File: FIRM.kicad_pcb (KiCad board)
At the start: 4 copper layers, 21.1 x 26.9 mm, 99 parts, among them J1 DM3CS-SF, J2 Conn_01x02_Pin, Q1 IRLML6402, U1 W25Q128JVS, U2 STM32F405RGTx, U3 ADXL371, U5 INA219AxDCN, U6 MIC5219-3.3YM5, U9 A-USBC-20F0-EA-GSR05, X1 32.768khz, Y1 12 MHz

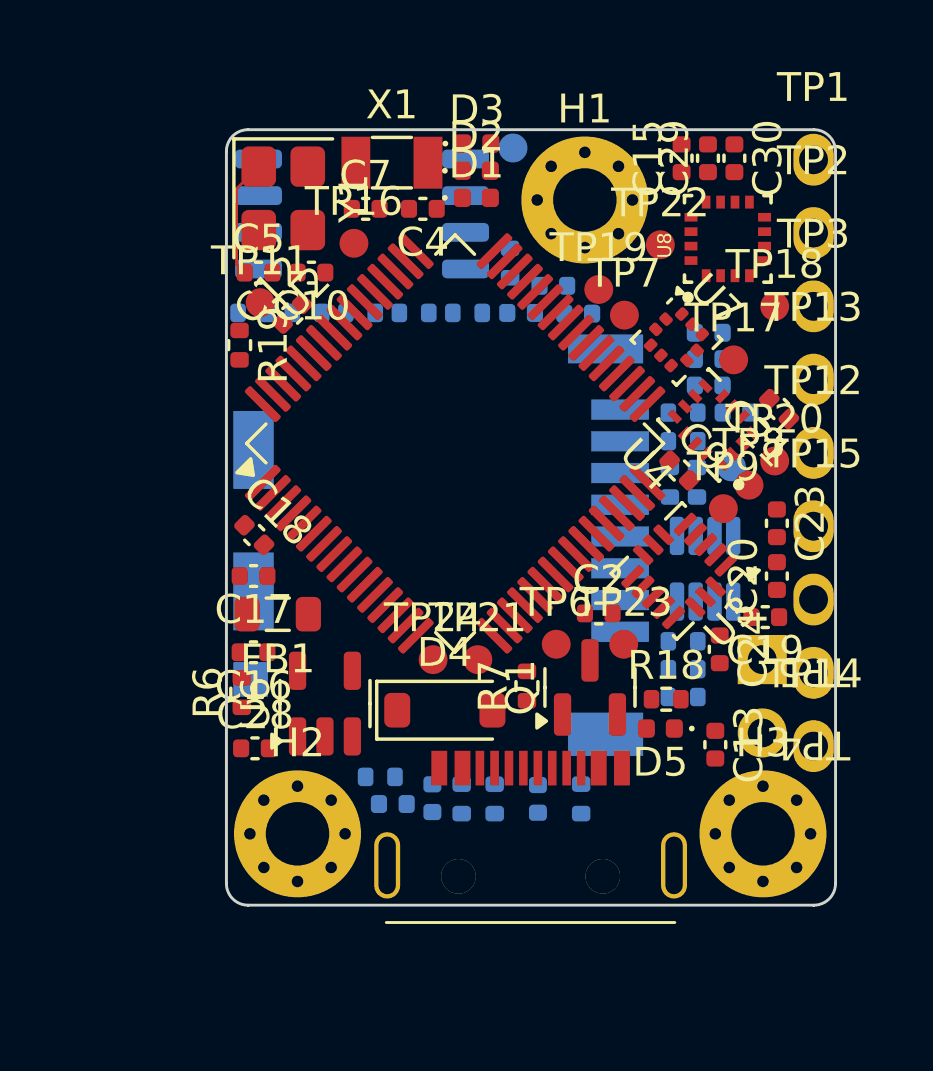
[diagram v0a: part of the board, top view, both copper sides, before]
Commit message: finished routing
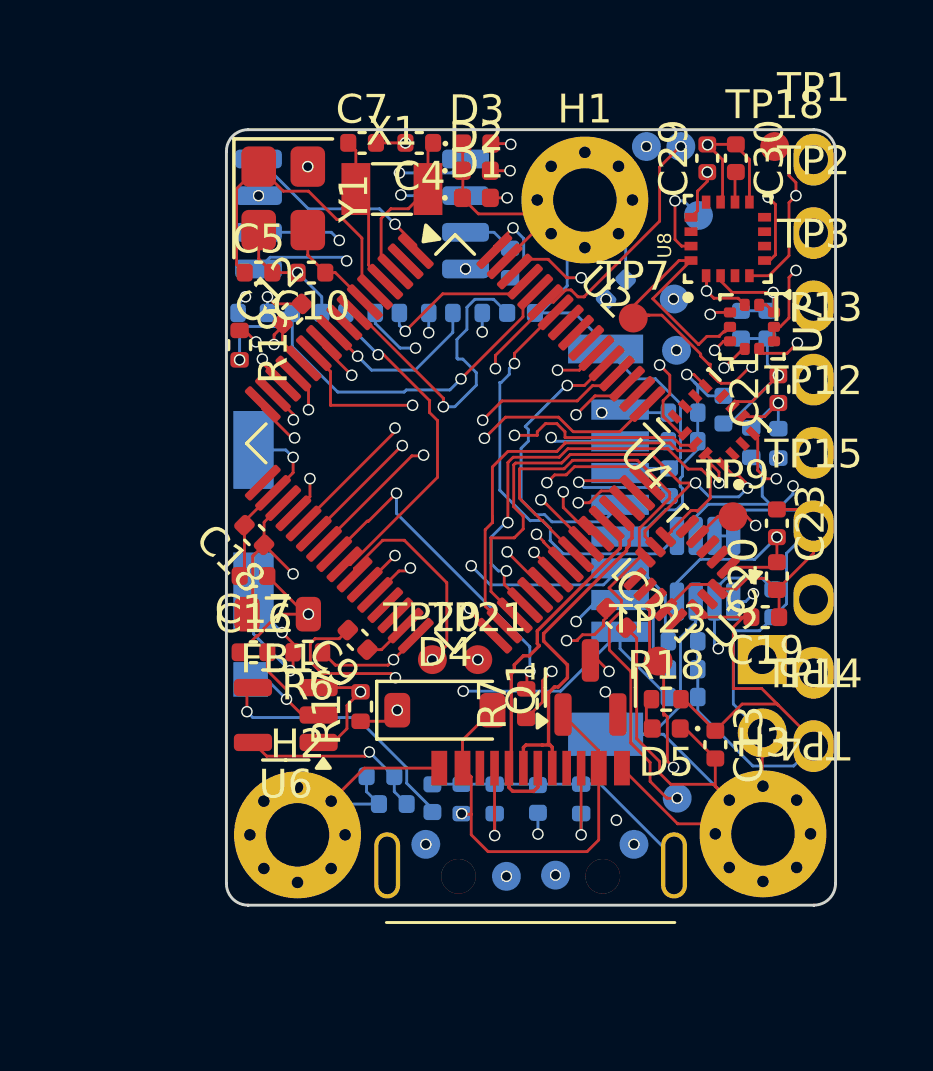
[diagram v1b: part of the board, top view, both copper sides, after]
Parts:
- removed C3, C6: 100n, Capacitor_SMD:C_0402_1005Metric
- C15, C24, C28, TP11, TP16, TP17, TP19, TP22, TP24, TP6, TP8: moved to B.Cu
- R17: moved to F.Cu
- moved TP25 25.2 mm to (163.1, 100.5)
- moved TP16 23.0 mm to (167.5, 99.4), turned to 180 degrees
- moved TP19 17.8 mm to (169.0, 97.8), turned to 180 degrees
- moved TP11 15.6 mm to (169.1, 75.3), turned to 180 degrees
- moved TP20 13.7 mm to (160.5, 93.0)
- moved C9 12.6 mm to (157.9, 92.4), turned to 135 degrees
- moved TP10 11.5 mm to (167.9, 75.3)
- moved TP24 8.59 mm to (164.8, 100.5), turned to 180 degrees
- moved TP6 8.28 mm to (160.3, 99.4), turned to 180 degrees
- moved TP8 6.95 mm to (168.9, 80.5), turned to 180 degrees
- moved C14 6.64 mm to (168.7, 86.9), turned to 90 degrees
- moved TP18 5.54 mm to (172.4, 75.3)
- moved C15 5.09 mm to (166.9, 80.2), turned to 45 degrees
- moved C28 4.45 mm to (158.7, 97.1), turned to 180 degrees
- moved R11 3.99 mm to (172.5, 85.5)
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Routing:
- net GND: track 0.00 -> 151.0 mm, vias 0 -> 12
- net +3.3V: track 0.00 -> 92.8 mm, vias 0 -> 17
- net /SCK2: track 0.00 -> 49.8 mm, vias 0 -> 3
- net /MISO2: track 0.00 -> 40.4 mm, vias 0 -> 5
- net /IMU_CS: track 0.00 -> 39.1 mm, vias 0 -> 3
- net /MOSI2: track 0.00 -> 37.8 mm, vias 0 -> 4
- net /I2C1_SCL: track 0.00 -> 35.1 mm, vias 0 -> 3
- net /BMP_INT: track 0.00 -> 31.5 mm, vias 0 -> 3
- net /I2C1_SDA: track 0.00 -> 31.0 mm, vias 0 -> 3
- net /NRST: track 0.00 -> 29.5 mm, vias 0 -> 2
- net /FLASH_CS: track 0.00 -> 27.1 mm, vias 0 -> 3
- net /MAG_CS: track 0.00 -> 25.8 mm, vias 0 -> 2
- net /IMU_INT: track 0.00 -> 25.7 mm, vias 0 -> 2
- net Net-(R19-Pad1): track 0.00 -> 24.2 mm, vias 0 -> 2
- net /SDIO_D2: track 0.00 -> 23.5 mm, vias 0 -> 2
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- added copper zone on In2.Cu, net +3.3V
- added copper zone on In1.Cu, net GND
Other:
- copper layers 4 -> 8

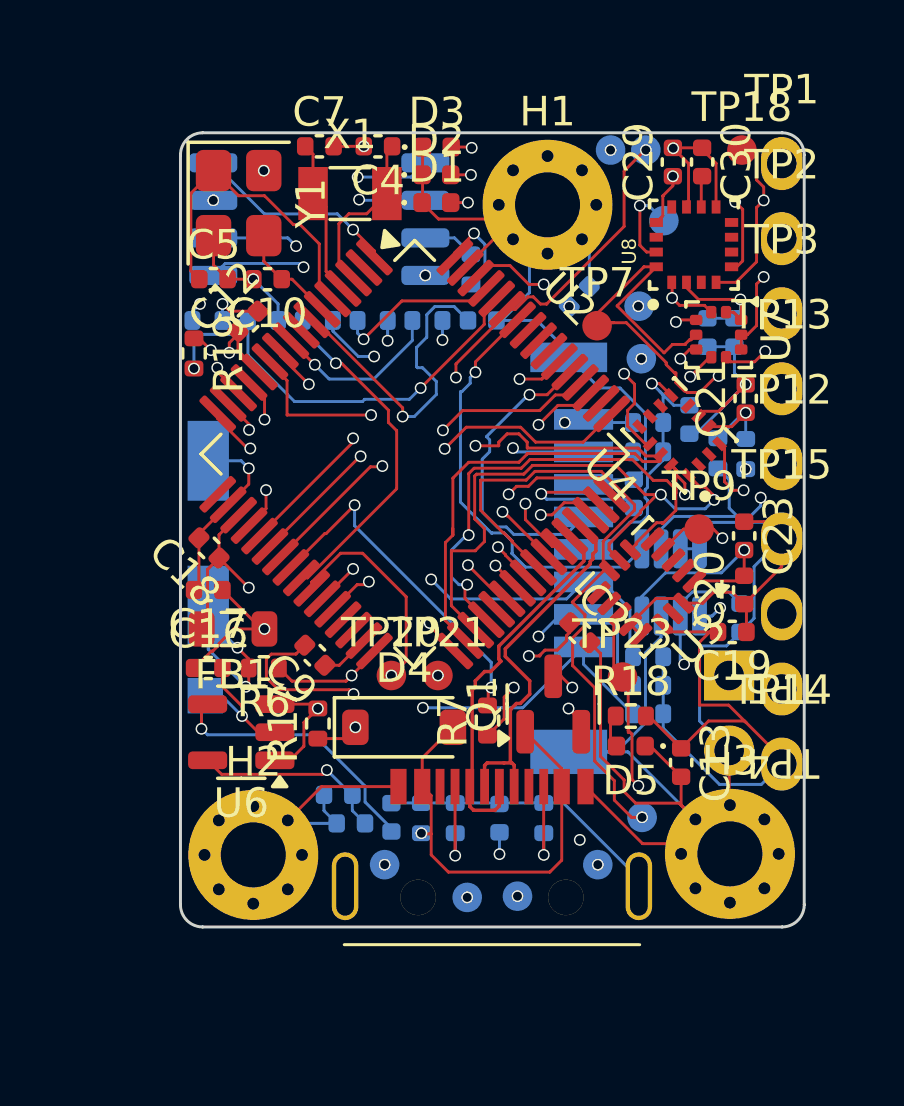
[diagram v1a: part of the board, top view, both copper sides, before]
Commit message: byebye drc errors
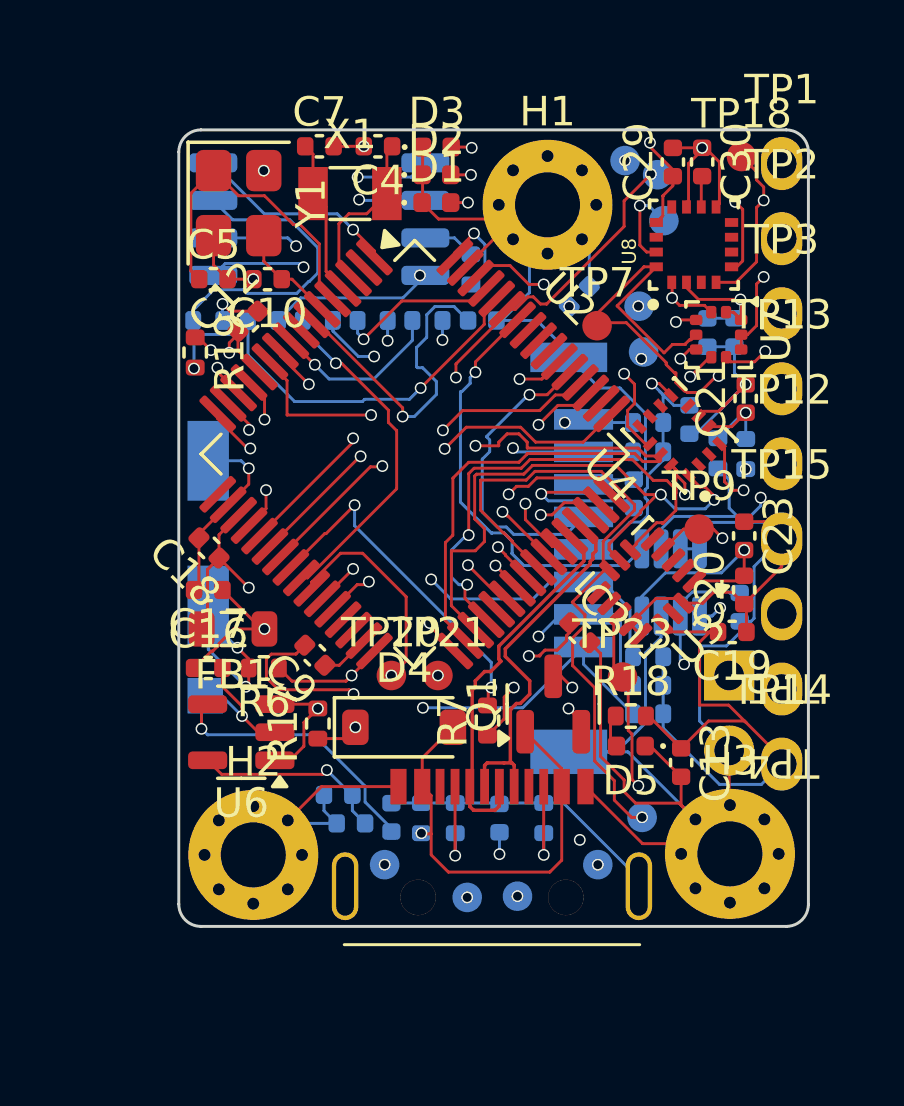
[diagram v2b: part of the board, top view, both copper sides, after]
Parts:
- moved TP11 0.93 mm to (169.5, 76.1)
- moved TP10 0.61 mm to (168.4, 75.6)
- moved C24 0.36 mm to (172.3, 90.7)
- moved TP17 0.24 mm to (169.1, 82.1)
- moved TP18 0.22 mm to (172.4, 75.5)
- moved R19 0.05 mm to (153.9, 82.1)
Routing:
- net Net-(U1-~{HOLD}/~{RESET}/IO_{3}): track 4.36 -> 10.6 mm, vias 2 -> 0
- net GND: track 151.0 -> 155.1 mm
- net +3.3V: track 92.8 -> 94.3 mm
- net /I2C1_SDA: track 31.0 -> 30.3 mm
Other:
- board size 21.1 x 26.9 mm -> 21.3 x 27 mm
